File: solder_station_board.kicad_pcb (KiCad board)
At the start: 2 copper layers, 104.8 x 60.3 mm, 34 parts, among them J1 Conn_01x04, J2 Conn_FB, J3 RT_WELLER, J4 VFD dISPLAY, J6 PWR_15V, P1 ISP, Q1 IRF9540, Q2 2N7002, U4 TLC272, U5 LT1007, U6 ATMEGA168-20AU, U7 HV5812-SOIC

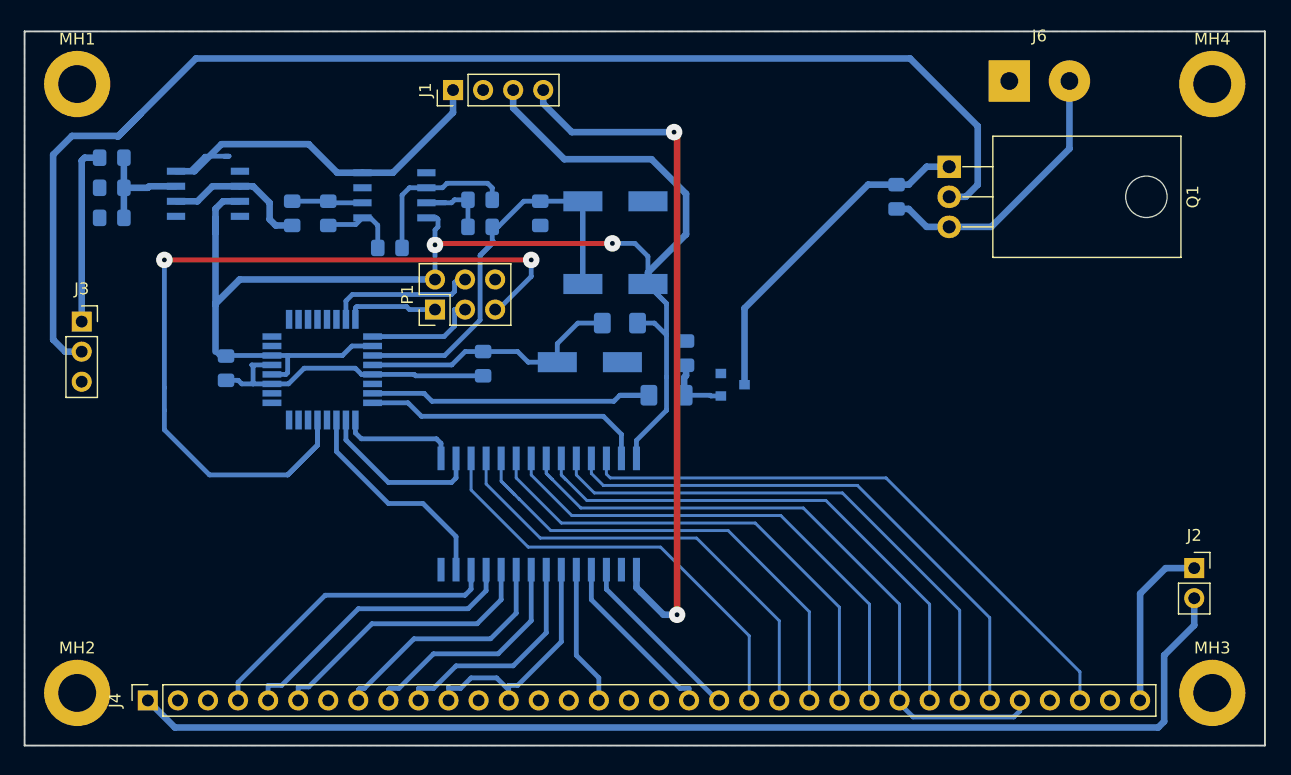
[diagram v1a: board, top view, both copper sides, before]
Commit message: Add inputs and refine
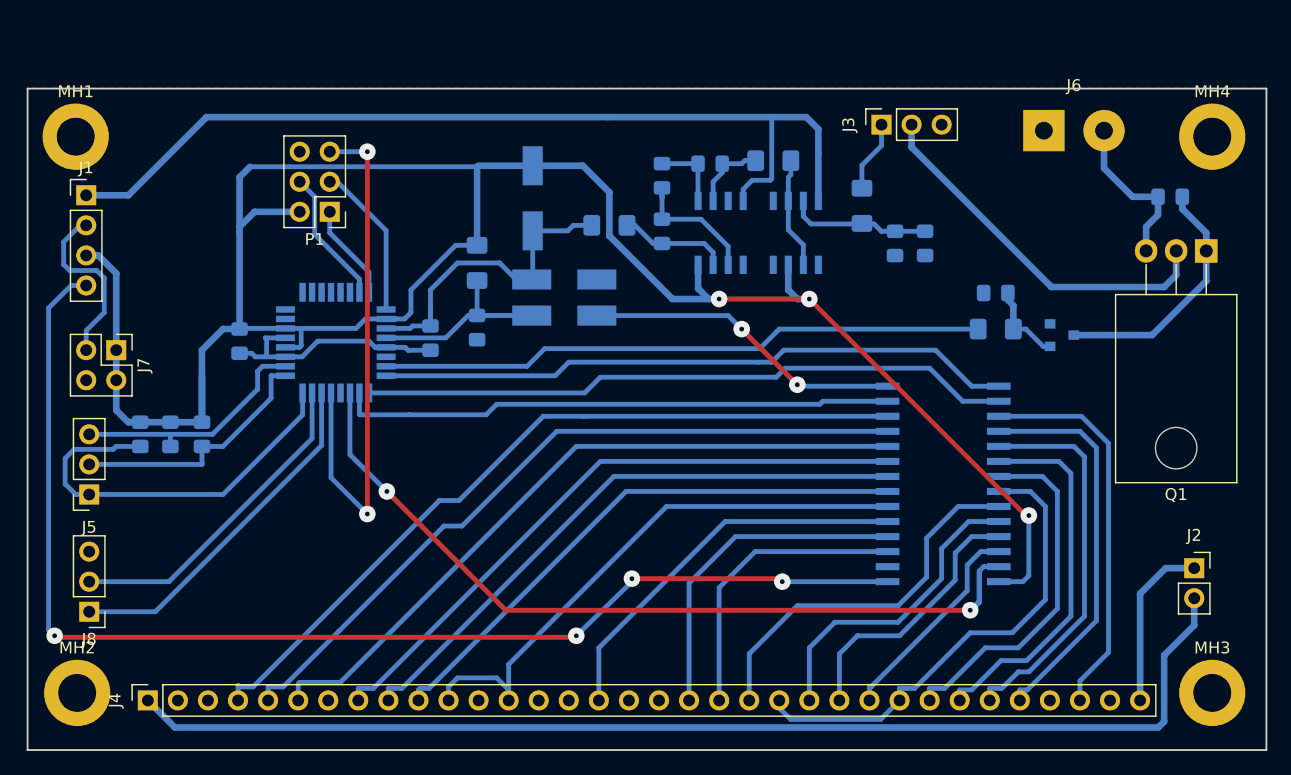
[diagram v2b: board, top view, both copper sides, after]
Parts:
- added J5: INPUT, Connector_PinSocket_2.54mm:PinSocket_1x03_P2.54mm_Vertical, F.Cu at (48.1, 68.0)
- added J7: INT_PWR, Connector_PinHeader_2.54mm:PinHeader_2x02_P2.54mm_Vertical, F.Cu at (50.4, 55.8)
- added J8: SERIAL, Connector_PinHeader_2.54mm:PinHeader_1x03_P2.54mm_Vertical, F.Cu at (48.1, 77.9)
- added R1: 1k, Resistor_SMD:R_0805_2012Metric_Pad1.15x1.40mm_HandSolder, B.Cu at (52.4, 62.9)
- added R2: 1k, Resistor_SMD:R_0805_2012Metric_Pad1.15x1.40mm_HandSolder, B.Cu at (57.6, 62.9)
- added R3: 1k, Resistor_SMD:R_0805_2012Metric_Pad1.15x1.40mm_HandSolder, B.Cu at (55.0, 62.9)
- J1: value Conn_01x04 -> PWR_5_36
- R10, R15, R5: footprint Resistor_SMD:R_0805_2012Metric_Pad1.15x1.40mm_HandSolder -> Resistor_SMD:R_1206_3216Metric_Pad1.42x1.75mm_HandSolder
- moved J3 69.6 mm to (115.0, 36.7), turned to 90 degrees
- moved C7 68.7 mm to (118.7, 46.8), turned to 270 degrees
- moved R7 66.3 mm to (116.2, 46.8), turned to 90 degrees
- moved R5 63.5 mm to (113.4, 43.6), turned to 90 degrees
- moved U5 49.8 mm to (107.8, 45.9), turned to 270 degrees
- moved R10 40.9 mm to (105.9, 39.8), turned to 180 degrees
- moved U7 34.3 mm to (120.2, 67.1), turned to 0 degrees
- moved R12 32.5 mm to (100.5, 40.0), turned to 180 degrees
- moved J1 32.2 mm to (47.8, 42.7), turned to 0 degrees
- moved R9 28.4 mm to (124.7, 54.0)
- moved Q2 28.1 mm to (130.3, 54.5)
- moved U4 27.7 mm to (101.4, 45.9), turned to 270 degrees
- moved R8 26.7 mm to (124.7, 51.0), turned to 0 degrees
- moved R13 23.8 mm to (96.5, 41.0), turned to 270 degrees
- moved R6 23.1 mm to (139.4, 42.8), turned to 0 degrees
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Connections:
- J4 pad 21: /f -> /b
- J4 pad 22: /e -> /1G
- J4 pad 23: /2G -> /a
- J4 pad 24: /d -> /S12
- J4 pad 25: /c -> /S10
- J4 pad 27: /b -> /c
- J4 pad 28: /a -> /d
- J4 pad 29: /S12 -> /2G
- J4 pad 30: /1G -> /e
- J4 pad 32: /S10 -> /f
- U6 pad 1: (no net) -> /INP2
- U6 pad 2: (no net) -> /INP3
- U6 pad 24: /SDI -> /CLOCK
- U6 pad 25: /CLOCK -> /STROBE
- U6 pad 26: /STROBE -> /BLANK
- U6 pad 27: /BLANK -> /SDI
- U6 pad 30: (no net) -> Net-(J8-Pad1)
- U6 pad 31: (no net) -> Net-(J8-Pad2)
- U6 pad 32: (no net) -> /INP1
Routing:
- net Net-(J3-Pad2): track 131.3 -> 31.6 mm
- net /SDI: track 25.4 -> 72.2 mm, vias 0 -> 2
- net -5V: track 35.2 -> 80.0 mm
- net +36V: track 60.5 -> 104.6 mm, vias 2 -> 4
- net /CLOCK: track 9.96 -> 53.9 mm
- net /STROBE: track 14.3 -> 55.2 mm
- net /S8: track 27.1 -> 65.7 mm
- net /7G: track 25.8 -> 62.4 mm
- net GND: track 26.0 -> 62.5 mm, vias 0 -> 2
- net /S7: track 23.9 -> 59.5 mm
- net /S10: track 52.1 -> 18.1 mm
- net /INP1: track 0.00 -> 34.0 mm
- net /6G: track 20.6 -> 53.7 mm
- net /S5: track 19.7 -> 50.6 mm
- net Net-(J8-Pad1): track 0.00 -> 29.9 mm
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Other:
- board size 104.8 x 60.3 mm -> 104.6 x 55.9 mm
